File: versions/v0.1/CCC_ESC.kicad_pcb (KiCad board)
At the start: 4 copper layers, 100 x 65 mm, 160 parts, among them J1 Conn_01x04, J2 Conn_01x04, J3 Conn_01x06, J4 Conn_01x06, U1 NCP5183, U2 NCP5183, U3 NCP5183, U4 NCS20074D, U5 STM32F401CCU6_Balckpill, U6 PQDE6W-Q110, U7 TO220_replacement_module

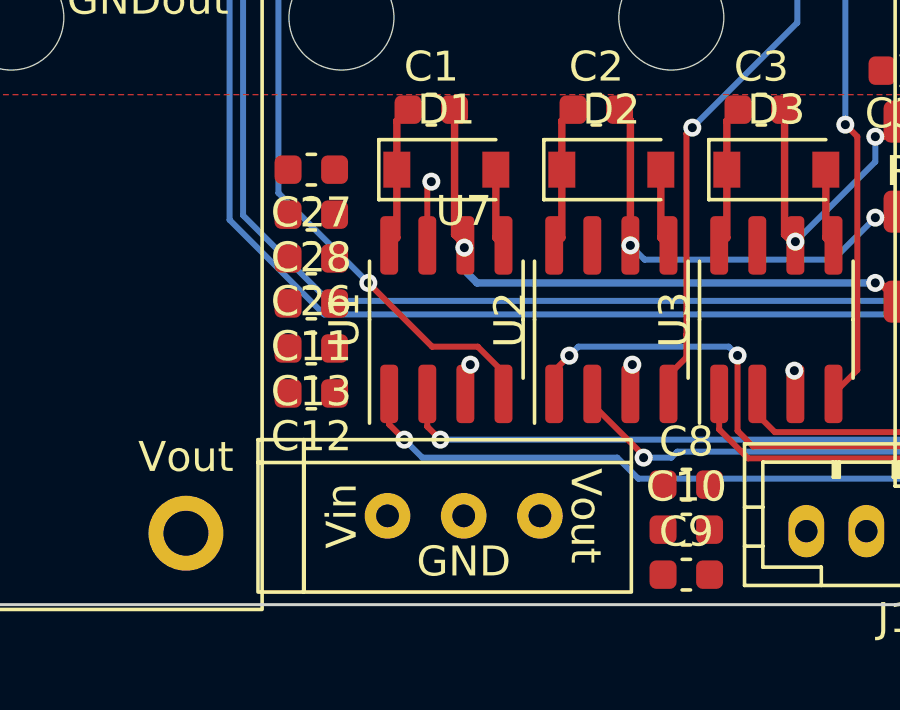
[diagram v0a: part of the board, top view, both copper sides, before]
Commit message: work in progress - pcb work tiny change
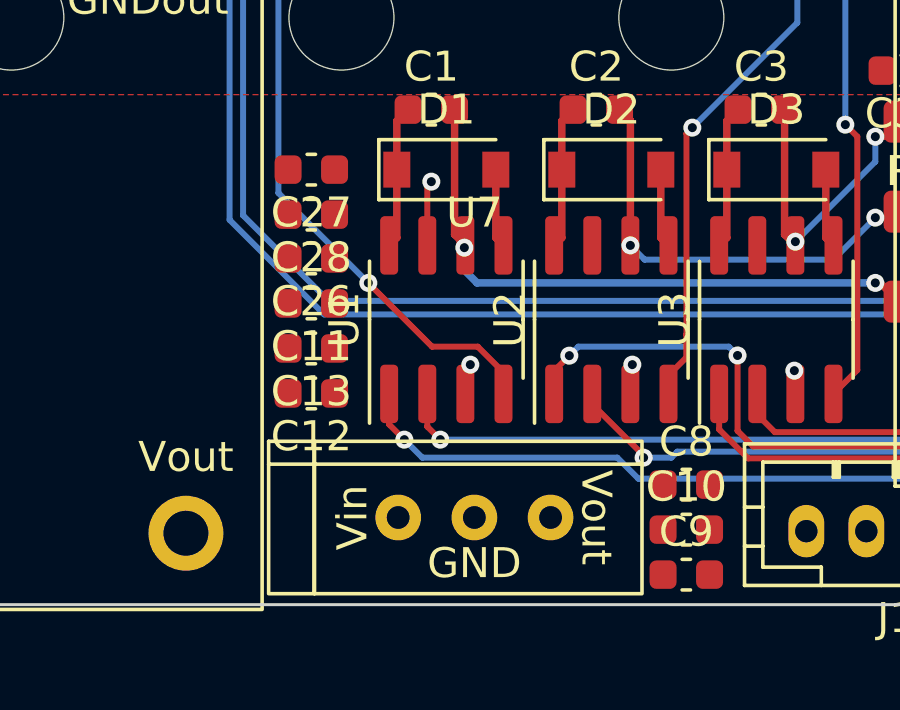
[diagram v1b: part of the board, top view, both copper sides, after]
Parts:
- moved U7 0.36 mm to (77.4, 109.6)
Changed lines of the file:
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@@
   )
   (footprint "CCC_ESC_Custom_parts:TO220_replacement_module" (layer "F.Cu")
-    (at 77 109.5)
+    (at 77.355 109.555)
     (property "Sheetfile" "CCC_ESC.kicad_sch")
     (property "Sheetname" "")
